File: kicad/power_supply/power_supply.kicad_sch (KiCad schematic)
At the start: 15 parts, among them J1 Conn_WallSocket_Earth, J2 Conn_01x03, J3 Conn_01x04_Pin, SW1 SW_SPST, T1 Transformer_SP_2S

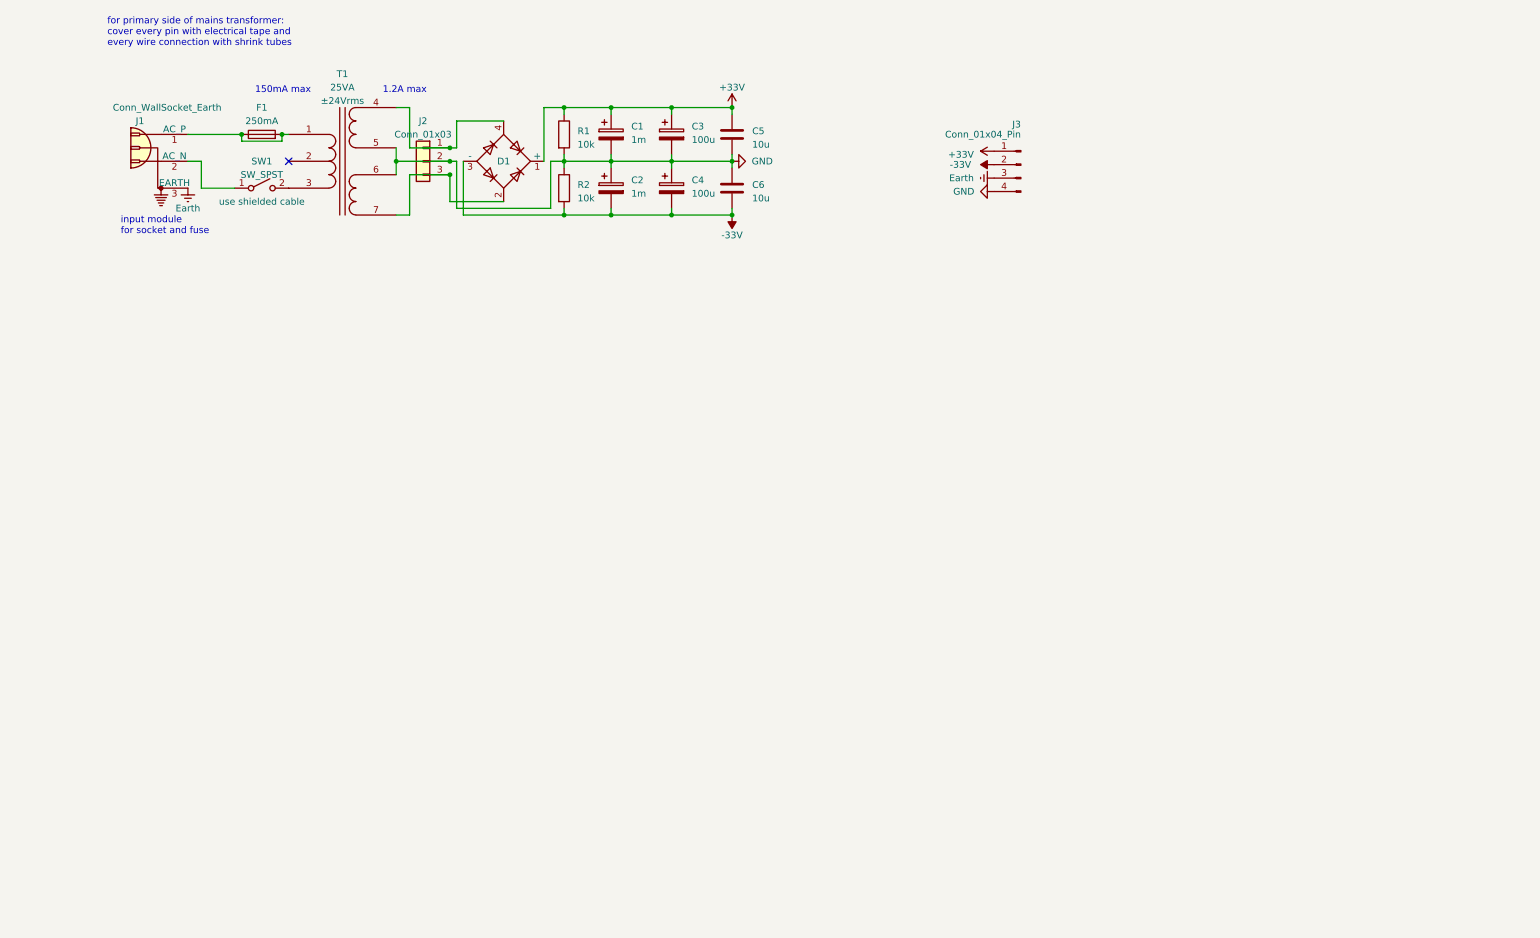
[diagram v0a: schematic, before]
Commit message: Commit
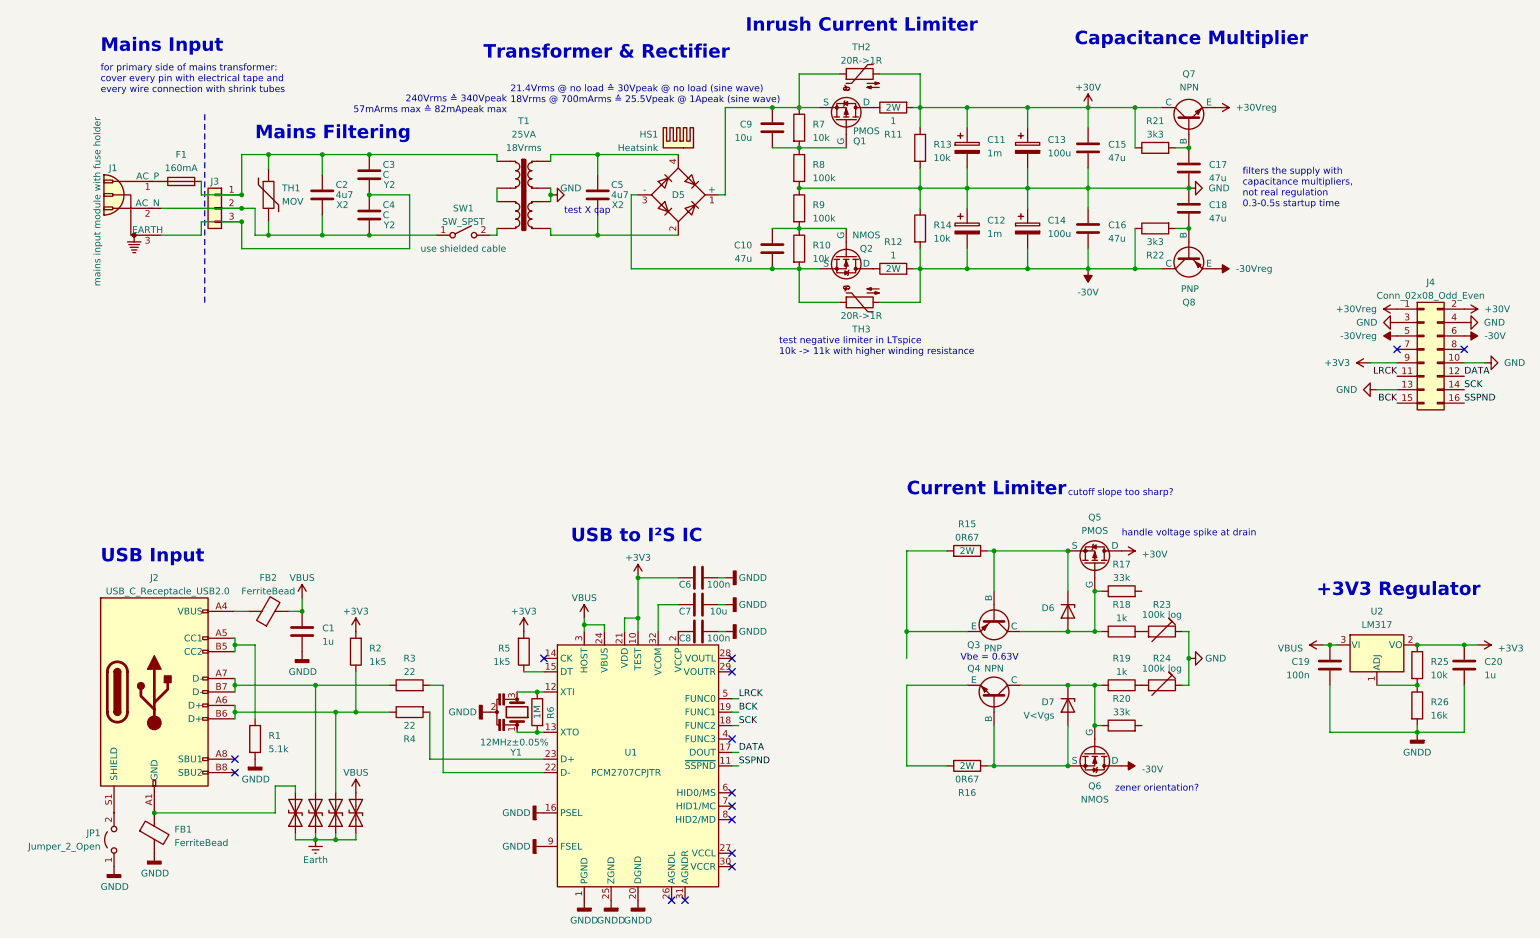
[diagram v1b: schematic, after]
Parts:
- removed J2: Conn_01x03, symbol Connector_Generic:Conn_01x03
- removed J3: Conn_01x04_Pin, symbol Connector:Conn_01x04_Pin
- added C1, C20: 1u, Capacitor_SMD:C_0805_2012Metric_Pad1.18x1.45mm_HandSolder, symbol Device:C
- added C10, C17, C18: 47u, Capacitor_SMD:C_0805_2012Metric_Pad1.18x1.45mm_HandSolder, symbol Device:C
- added C19, C6, C8: 100n, Capacitor_SMD:C_0805_2012Metric_Pad1.18x1.45mm_HandSolder, symbol Device:C
- added C2, C5: 4u7, symbol Device:C
- added C3, C4: C, symbol Device:C
- added C7, C9: 10u, Capacitor_SMD:C_0805_2012Metric_Pad1.18x1.45mm_HandSolder, symbol Device:C
- added D1, D2, D3, D4: D_TVS, symbol Device:D_TVS
- added D6, D7: V<Vgs, symbol Device:D_Zener
- added FB1, FB2: FerriteBead, symbol Device:FerriteBead
- added HS1: Heatsink, symbol Mechanical:Heatsink
- added J2: USB_C_Receptacle_USB2.0, Connector_USB:USB_C_Receptacle_GCT_USB4085, symbol Connector:USB_C_Receptacle_USB2.0
- added J3: Conn_01x03, symbol Connector_Generic:Conn_01x03
- added J4: Conn_02x08_Odd_Even, Connector_PinSocket_2.54mm:PinSocket_2x08_P2.54mm_Vertical, symbol Connector_Generic:Conn_02x08_Odd_Even
- added JP1: Jumper_2_Open, Jumper:SolderJumper-2_P1.3mm_Open_Pad1.0x1.5mm, symbol Jumper:Jumper_2_Open
- added Q1, Q5: PMOS, symbol Simulation_SPICE:PMOS
- added Q2, Q6: NMOS, symbol Simulation_SPICE:NMOS
- added Q3: PNP, symbol Simulation_SPICE:PNP
- added Q4: NPN, symbol Simulation_SPICE:NPN
- added Q7: NPN, Package_TO_SOT_THT:TO-220-3_Vertical, symbol Simulation_SPICE:NPN
- added Q8: PNP, Package_TO_SOT_THT:TO-220-3_Vertical, symbol Simulation_SPICE:PNP
- added R1: 5.1k, Resistor_SMD:R_0805_2012Metric_Pad1.20x1.40mm_HandSolder, symbol Device:R
- added R10, R25, R7: 10k, Resistor_SMD:R_0805_2012Metric_Pad1.20x1.40mm_HandSolder, symbol Device:R
- added R11, R12: 1, symbol Device:R
- added R15, R16: 0R67, symbol Device:R
- added R17, R20: 33k, Resistor_SMD:R_0805_2012Metric_Pad1.20x1.40mm_HandSolder, symbol Device:R
- added R18, R19: 1k, Resistor_SMD:R_0805_2012Metric_Pad1.20x1.40mm_HandSolder, symbol Device:R
- added R2, R5: 1k5, Resistor_SMD:R_0805_2012Metric_Pad1.20x1.40mm_HandSolder, symbol Device:R
- added R21, R22: 3k3, Resistor_SMD:R_0805_2012Metric_Pad1.20x1.40mm_HandSolder, symbol Device:R
- added R23, R24: 100k log, symbol Device:R_Trim
- added R26: 16k, Resistor_SMD:R_0805_2012Metric_Pad1.20x1.40mm_HandSolder, symbol Device:R
- added R3, R4: 22, Resistor_SMD:R_0805_2012Metric_Pad1.20x1.40mm_HandSolder, symbol Device:R
- added R6: 1M, Resistor_SMD:R_0805_2012Metric_Pad1.20x1.40mm_HandSolder, symbol Device:R
- added R8, R9: 100k, Resistor_SMD:R_0805_2012Metric_Pad1.20x1.40mm_HandSolder, symbol Device:R
- added TH1: MOV, symbol Device:Thermistor
- added TH2, TH3: 20R->1R, Capacitor_THT:C_Disc_D9.0mm_W5.0mm_P5.00mm, symbol Device:Thermistor_NTC
- added U1: PCM2707CPJTR, Package_QFP:TQFP-32_7x7mm_P0.8mm, symbol library:PCM2707CPJTR
- added U2: LM317, Package_TO_SOT_SMD:SOT-89-3, symbol Regulator_Linear:LM317L_SOT-89
- added Y1: 12MHz±0.05%, symbol Device:Resonator
- C15: renamed from C5; value 10u -> 47u
- C16: renamed from C6; value 10u -> 47u
- F1: value 250mA -> 160mA; Digikey 507-2270-ND -> 507-1238-ND
- J1: Note (none) -> mains input module with fuse holder
- T1: symbol Device:Transformer_SP_2S -> Transformer:TRANSF6; Digikey 237-1328-ND -> 1295-1074-ND; Spannung ±24Vrms -> 18Vrms
- renumbered C1 to C11, C2 to C12, C3 to C13, C4 to C14, D1 to D5, R1 to R13, R2 to R14
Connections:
- net Earth: now also D1.1 (A1), D2.1 (A1), D3.1 (A1), D4.1 (A1); no longer J1.3 (EARTH)
- net GND: now also T1.7, C17.2, C18.1, J4.10 (Pin_10), J4.13 (Pin_13), J4.3 (Pin_3), J4.4 (Pin_4), R23.1, R24.1, R8.2, R9.1; no longer T1.5 (OUT1B)
- net at F1.1, J1.1 (AC_P): no longer F1.2, T1.1 (IN+)
- net at J1.2 (AC_N), SW1.1 (A): now also C2.2, C4.2, J3.2 (Pin_2), TH1.2
- net at D5.2: now also T1.5, C5.2; no longer T1.7 (OUT2B)
- net at D5.4: now also T1.8, C5.1; no longer T1.4 (OUT1A)
- net at SW1.2 (B): now also T1.4; no longer T1.3 (IN-)
- net at T1.2: now also T1.3
- net +36V renamed +30V
- net +30V: now also J4.2 (Pin_2), Q5.1 (D), Q7.1 (C), R11.2, R21.1, TH2.2; no longer D5.1 (+)
- net -36V renamed -30V
- net -30V: now also J4.6 (Pin_6), Q6.1 (D), Q8.1 (C), R12.2, R22.1, TH3.2; no longer D5.3 (-)
- new net: C18.2, Q8.2 (B), R22.2
- new net: D6.1 (K), Q3.2 (B), Q5.3 (S), R15.1
- new net: D6.2 (A), Q3.1 (C), Q5.2 (G), R17.1, R18.1
- new net: C17.1, Q7.2 (B), R21.2
- new net: R6.2, U1.13 (XTO), Y1.1
- new net: R6.1, U1.12 (XTI), Y1.3
- new net: R5.1, U1.15 (DT)
- new net: C3.2, C4.1, J1.3 (EARTH), J3.3 (Pin_3)
- new net: R25.2, R26.1, U2.1 (ADJ)
- new net: D2.2 (A2), J2.A7 (D-), J2.B7 (D-), R3.1
- new net: C9.1, D5.1 (+), Q1.3 (S), R7.1, TH2.1
- new net: C9.2, Q1.2 (G), R7.2, R8.1
- new net: R19.1, R24.2
- new net: D7.1 (K), Q4.1 (C), Q6.2 (G), R19.2, R20.1
- new net: C2.1, C3.1, F1.2, J3.1 (Pin_1), T1.1, TH1.1
- new net: Q3.3 (E), R15.2
- new net: Q1.1 (D), R11.1
- new net: D3.2 (A2), J2.A6 (D+), J2.B6 (D+), R2.1, R4.1
- new net: D1.2 (A2), FB1.1, J2.A1 (GND), J2.A12 (GND), J2.B1 (GND), J2.B12 (GND)
- new net: FB2.1, J2.A4 (VBUS), J2.A9 (VBUS), J2.B4 (VBUS), J2.B9 (VBUS)
- new net: J2.A5 (CC1), J2.B5 (CC2), R1.1
- new net: J2.S1 (SHIELD), JP1.2 (B)
- new net: C10.1, Q2.2 (G), R10.1, R9.2
- new net: C10.2, D5.3 (-), Q2.3 (S), R10.2, TH3.1
- new net: C8.2, U1.2 (VCCP)
- new net: R3.2, U1.22 (D-)
- new net: R4.2, U1.23 (D+)
- new net: C7.2, U1.32 (VCOM)
- new net: Q2.1 (D), R12.1
- new net: D7.2 (A), Q4.2 (B), Q6.3 (S), R16.1
- new net: Q4.3 (E), R16.2
- new net: R18.2, R23.2
- new net +30Vreg: J4.1 (Pin_1), Q7.3 (E)
- new net +3V3: C20.2, C6.2, J4.9 (Pin_9), R2.2, R25.1, R5.2, U1.10 (TEST), U1.21 (VDD), U2.2 (VO)
- new net -30Vreg: J4.5 (Pin_5), Q8.3 (E)
- new net BCK: J4.15 (Pin_15), U1.19 (FUNC1)
- new net DATA: J4.12 (Pin_12), U1.17 (DOUT)
- new net GNDD: C1.1, C19.1, C20.1, C6.1, C7.1, C8.1, FB1.2, JP1.1 (A), R1.2, R26.2, U1.1 (PGND), U1.16 (PSEL), U1.20 (DGND), U1.25 (ZGND), U1.9 (FSEL), Y1.2
- new net LRCK: J4.11 (Pin_11), U1.5 (FUNC0)
- new net SCK: J4.14 (Pin_14), U1.18 (FUNC2)
- new net SSPND: J4.16 (Pin_16), U1.11 (~{SSPND})
- new net VBUS: C1.2, C19.2, D4.2 (A2), FB2.2, U1.24 (VBUS), U1.3 (HOST), U2.3 (VI)
- no-connect marks 1 -> 15
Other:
- note added: "+3V3 Regulator"
- note added: "21.4Vrms @ no load ≙ 30Vpeak @ no load (sine wave) 18Vrms @ 700mArms ≙ 25.5Vpeak @ 1Apeak (sine wave)"
- note added: "240Vrms ≙ 340Vpeak 57mArms max ≙ 82mApeak max"
- note added: "Capacitance Multiplier"
- note added: "Current Limiter"
- note added: "Inrush Current Limiter"
- note added: "Mains Filtering"
- note added: "Mains Input"
- note added: "Transformer & Rectifier"
- note added: "USB Input"
- note added: "USB to I²S IC"
- note added: "Vbe = 0.63V"
- note added: "cutoff slope too sharp?"
- note added: "filters the supply with capacitance multipliers, not real regulation 0.3-0.5s startup time"
- note added: "handle voltage spike at drain"
- note added: "test X cap"
- note added: "test negative limiter in LTspice 10k -> 11k with higher winding resistance"
- note added: "zener orientation?"
- note removed: "1.2A max"
- note removed: "150mA max"
- note removed: "input module for socket and fuse"
- moved on the sheet: C11, C12, C13, C14, C15, C16, D5, J1, R13, R14, SW1
